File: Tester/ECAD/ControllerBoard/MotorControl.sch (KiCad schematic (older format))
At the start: 18 parts, among them J2 Conn_01x02_Male, J3 Conn_01x02_Male, J4 Conn_01x02_Male, J5 Conn_01x02_Male, U3 DRV8833PW, U4 DRV8833PW

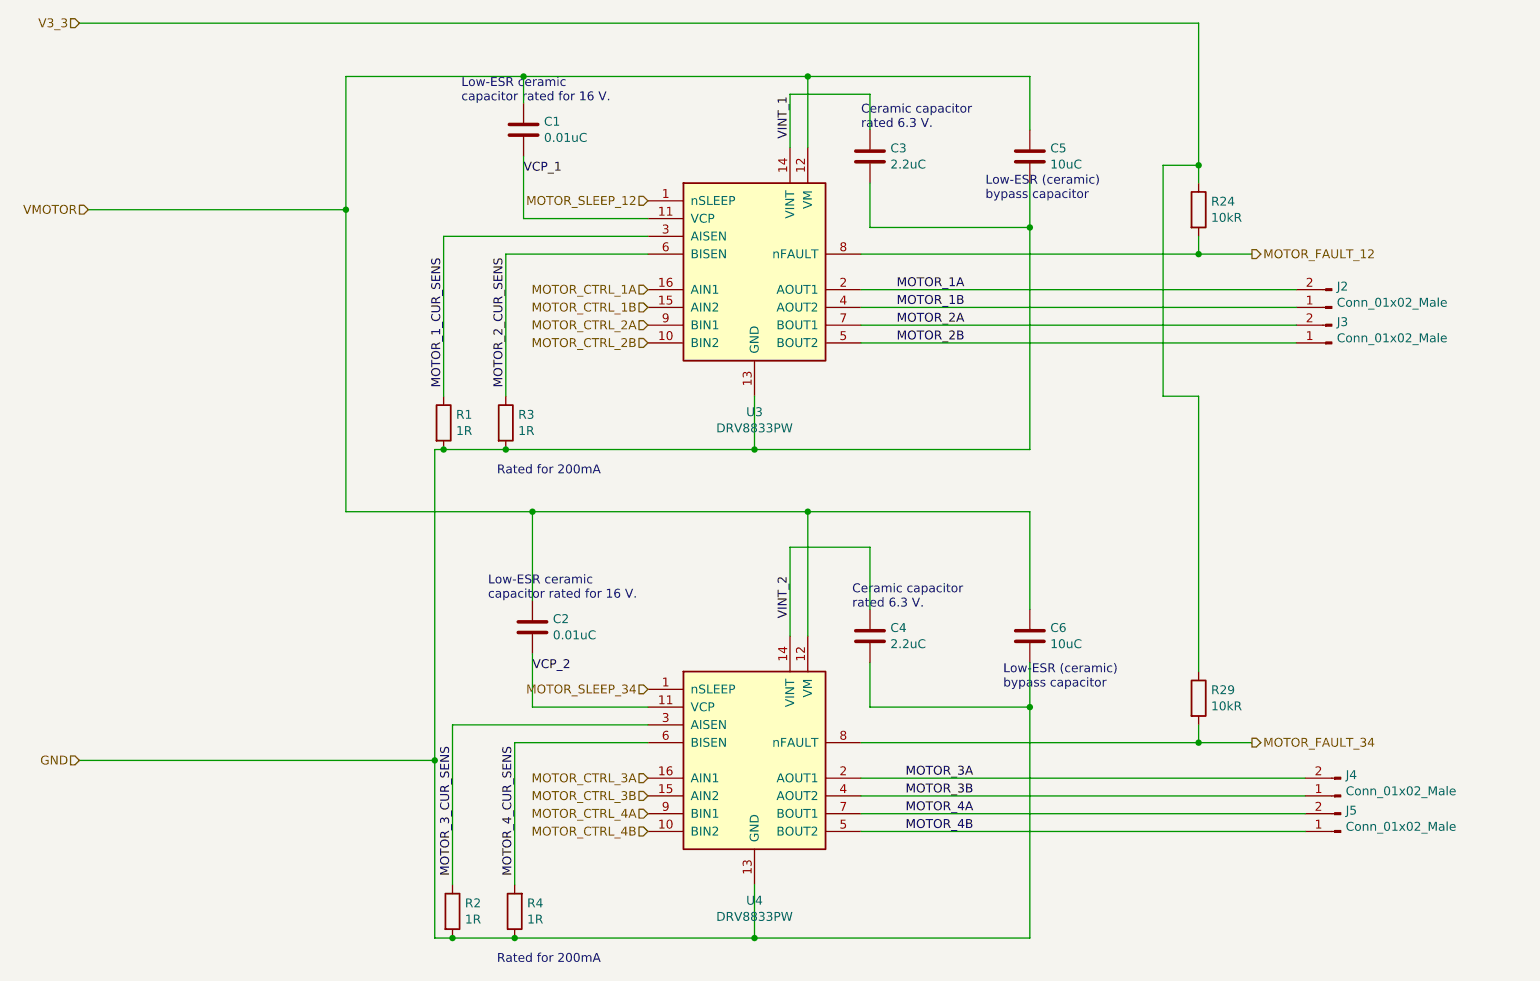
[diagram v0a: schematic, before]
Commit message: Progressed circuit updates.
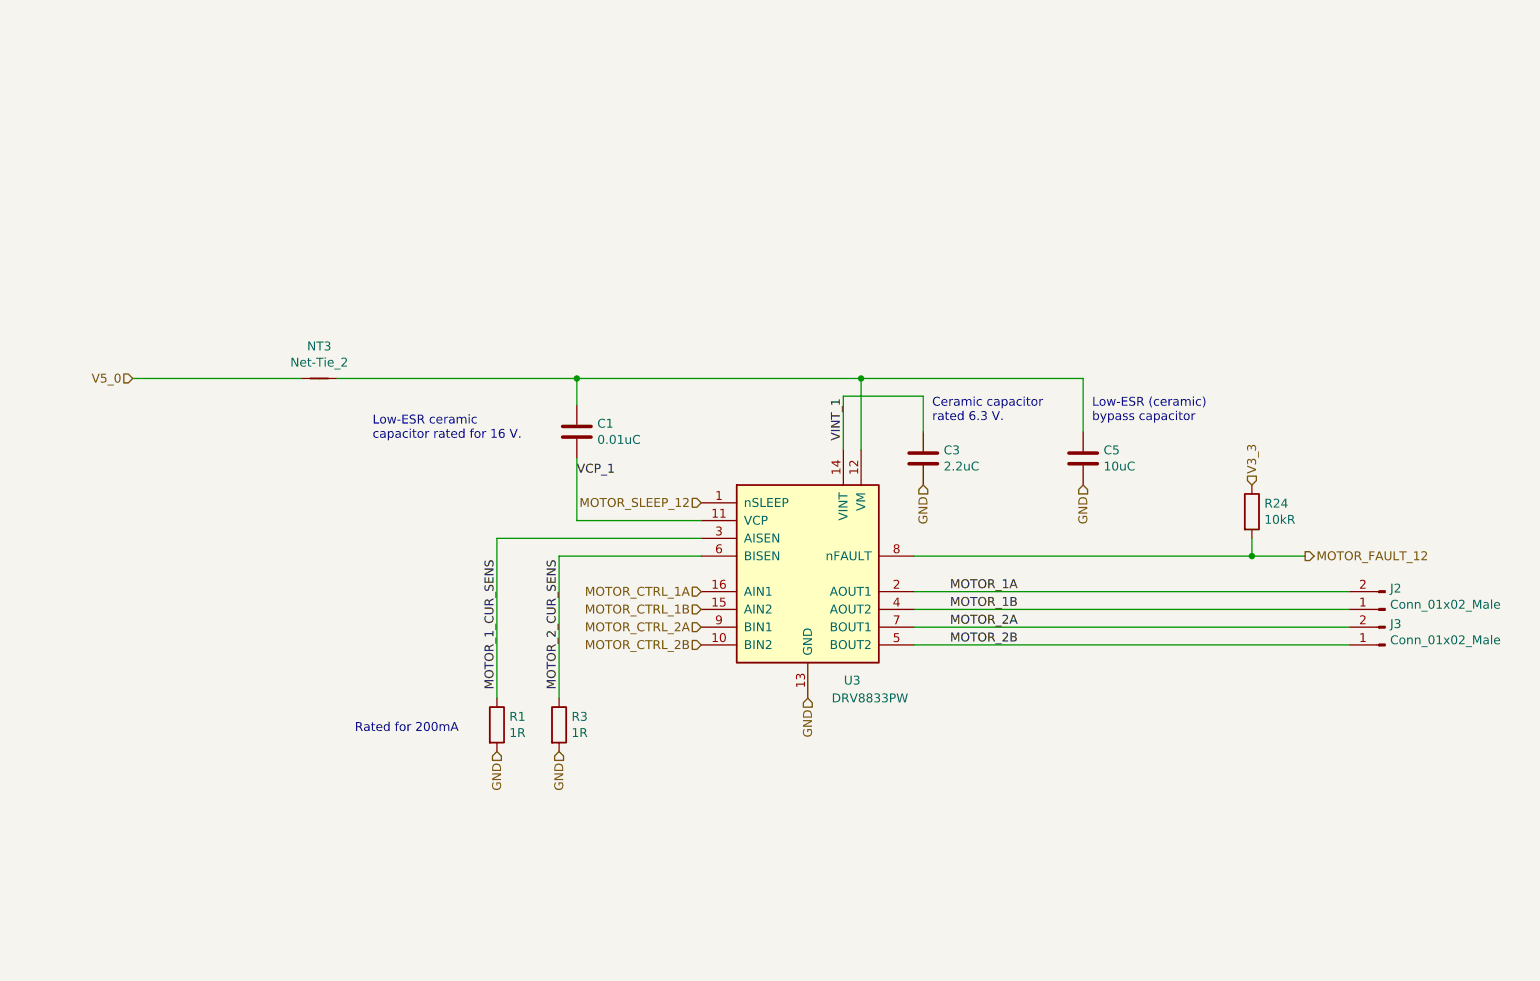
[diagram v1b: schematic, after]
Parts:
- removed C2: 0.01uC, Capacitor_SMD:C_0805_2012Metric_Pad1.15x1.40mm_HandSolder, symbol Device:C
- removed C4: 2.2uC, Capacitor_SMD:C_0805_2012Metric_Pad1.15x1.40mm_HandSolder, symbol Device:C
- removed C6: 10uC, Capacitor_SMD:C_0805_2012Metric_Pad1.15x1.40mm_HandSolder, symbol Device:C
- removed J4, J5: Conn_01x02_Male, symbol Connector:Conn_01x02_Male
- removed R2, R4: 1R, Resistor_SMD:R_0805_2012Metric_Pad1.15x1.40mm_HandSolder, symbol Device:R
- removed R29: 10kR, Resistor_SMD:R_0805_2012Metric_Pad1.15x1.40mm_HandSolder, symbol Device:R
- removed U4: DRV8833PW, Package_SO:TSSOP-16_4.4x5mm_P0.65mm, symbol Driver_Motor:DRV8833PW
- added NT3: Net-Tie_2, symbol Device:Net-Tie_2
- J2, J3: footprint (none) -> Connector_JST:JST_XH_B2B-XH-A_1x02_P2.50mm_Vertical; Manufacturer Part Number (none) -> B2B-XH-A(LF)(SN)
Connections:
- net VMOTOR: no longer names the net of C1.1, C5.1, U3.12 (VM)
- net VMOTOR: now also NT3.2
- new net V5_0: NT3.1
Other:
- moved on the sheet: C1, C3, C5, J2, J3, R1, R24, R3, U3
